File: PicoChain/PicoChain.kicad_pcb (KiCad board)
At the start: 2 copper layers, 14 parts, among them J1 RJ45, J2 RJ45, J3 Conn_01x02_Socket, J4 Conn_01x02_Socket, J5 Conn_01x20_Socket, J6 Conn_01x20_Socket, U1 PCA9615DP, U2 RASPBERRY_PI_PICO

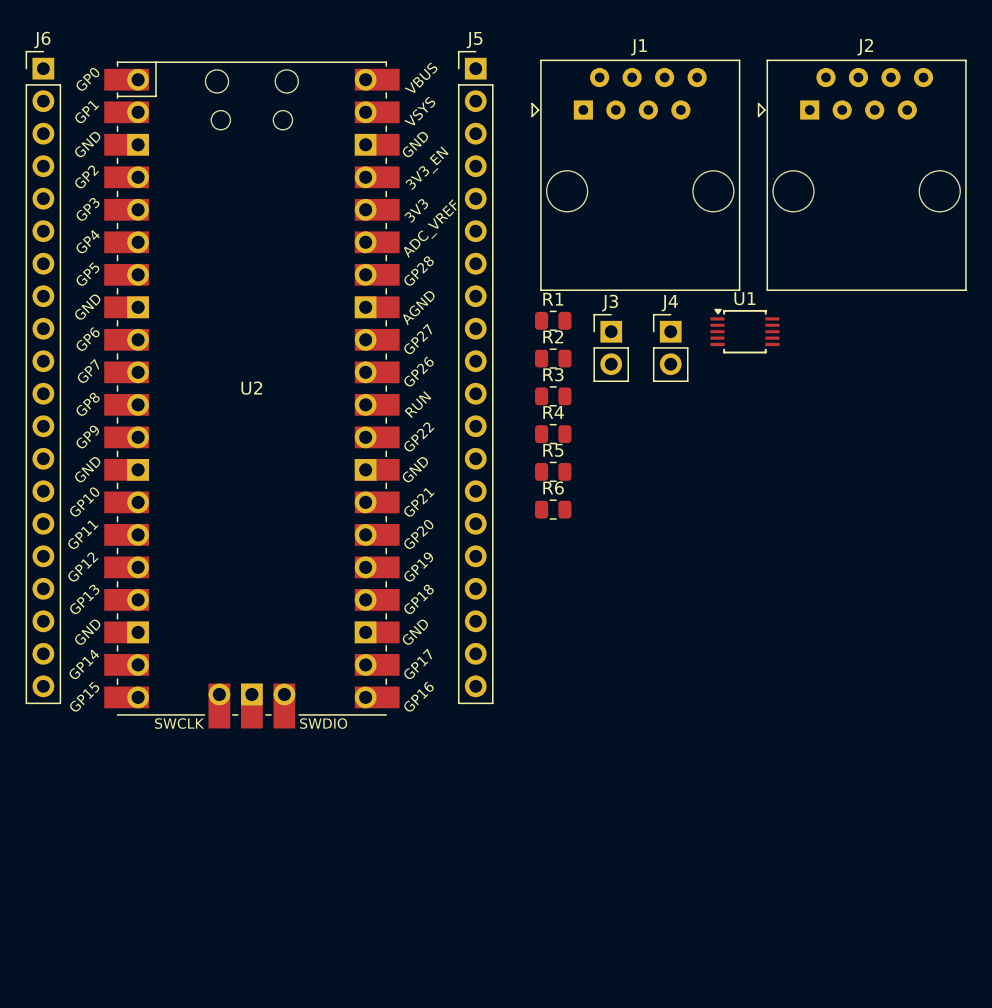
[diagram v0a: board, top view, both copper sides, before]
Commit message: Updated to version 1.1
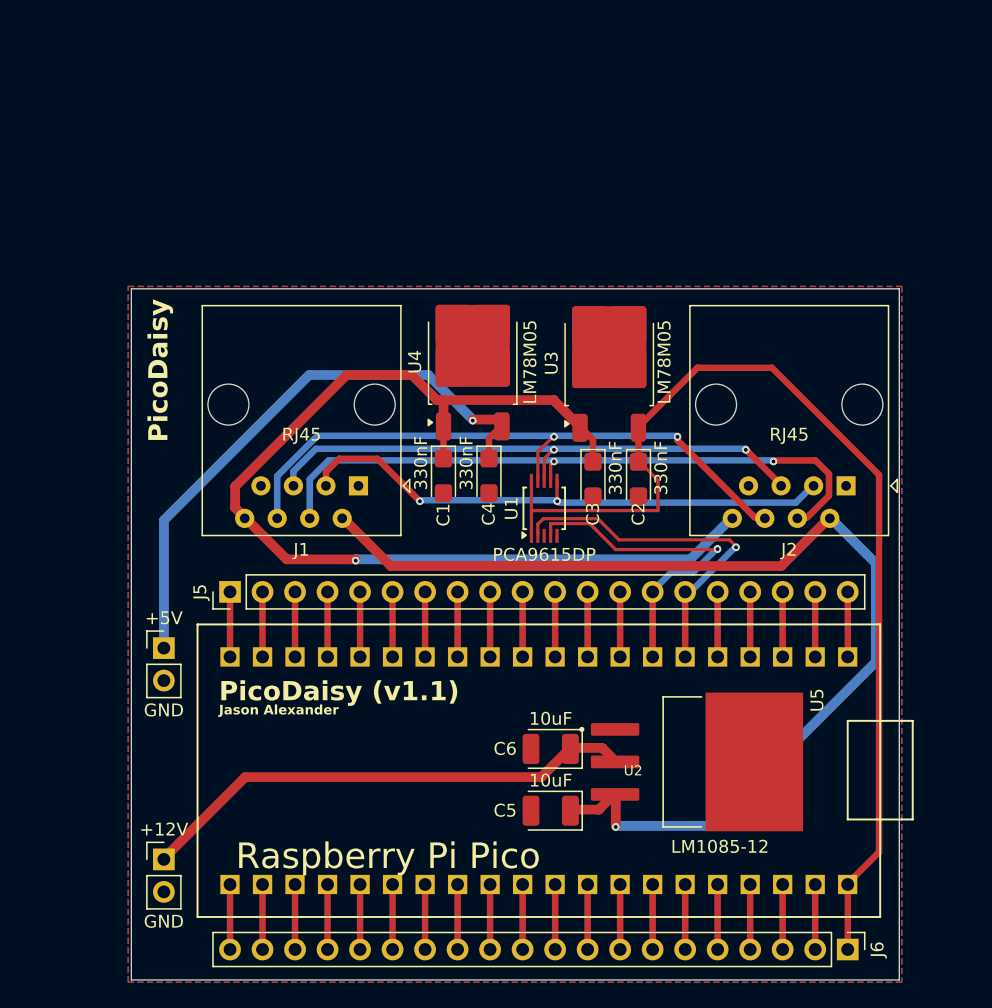
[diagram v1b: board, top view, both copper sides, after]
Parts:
- removed J3, J4: Conn_01x02_Socket, Connector_PinHeader_2.54mm:PinHeader_1x02_P2.54mm_Vertical
- removed R1, R3, R4, R6: 470, Resistor_SMD:R_0805_2012Metric
- removed R2, R5: 140, Resistor_SMD:R_0805_2012Metric
- added +12V: GND, Connector_PinHeader_2.54mm:PinHeader_1x02_P2.54mm_Vertical, F.Cu at (128.5, 112.6)
- added +5V: GND, Connector_PinHeader_2.54mm:PinHeader_1x02_P2.54mm_Vertical, F.Cu at (128.5, 96.1)
- added C1: 330nF, Capacitor_Tantalum_SMD:CP_EIA-3216-18_Kemet-A, F.Cu at (150.4, 82.6)
- added C2: 330nF, Capacitor_Tantalum_SMD:CP_EIA-3216-18_Kemet-A, F.Cu at (165.6, 82.9)
- added C3: 330nF, Capacitor_Tantalum_SMD:CP_EIA-3216-18_Kemet-A, F.Cu at (162.1, 82.9)
- added C4: 330nF, Capacitor_Tantalum_SMD:CP_EIA-3216-18_Kemet-A, F.Cu at (153.9, 82.6)
- added C5: 10uF, Capacitor_Tantalum_SMD:CP_EIA-3528-21_Kemet-B, F.Cu at (158.8, 108.8)
- added C6: 10uF, Capacitor_Tantalum_SMD:CP_EIA-3528-21_Kemet-B, F.Cu at (158.8, 104.0)
- added U3: LM78M05, Package_TO_SOT_SMD:TO-252-2, F.Cu at (163.3, 73.8)
- added U4: LM78M05, Package_TO_SOT_SMD:TO-252-2, F.Cu at (152.7, 73.7)
- added U5: LM1085-12, LM1085IS-12:TO254P1524X483-4N, F.Cu at (170.2, 105.0)
- U2: footprint MCU_RaspberryPi_and_Boards:RPi_Pico_SMD_TH -> RASPBERRY_PI_PICO:RASPBERRY_PI_PICO
- moved J6 93.2 mm to (182.0, 119.6), turned to -90 degrees
- moved J5 45.2 mm to (133.7, 91.7), turned to 90 degrees
- moved U2 38.1 mm to (159.1, 105.7), turned to -90 degrees
- moved J1 34.2 mm to (143.7, 83.4), turned to 180 degrees
- moved J2 29.5 mm to (181.8, 83.4), turned to 180 degrees
- moved U1 20.9 mm to (158.3, 85.2), turned to 90 degrees
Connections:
- J1 pad 1: Net-(U1-DSCLM) -> GND
- J1 pad 2: Net-(U1-DSCLP) -> +24V
- J1 pad 3: +5V -> Net-(U1-DSCLM)
- J1 pad 4: GND -> Net-(U1-DSCLP)
- J1 pad 5: /+5V(M) -> Net-(U1-DSDAP)
- J1 pad 6: +12V -> Net-(U1-DSDAM)
- J1 pad 7: Net-(U1-DSDAM) -> GND
- J1 pad 8: Net-(U1-DSDAP) -> +12V
- J2 pad 1: Net-(U1-DSCLM) -> GND
- J2 pad 2: Net-(U1-DSCLP) -> +24V
- J2 pad 3: +5V -> Net-(U1-DSCLM)
- J2 pad 4: GND -> Net-(U1-DSCLP)
- J2 pad 5: /+5V(M) -> Net-(U1-DSDAP)
- J2 pad 6: +12V -> Net-(U1-DSDAM)
- J2 pad 7: Net-(U1-DSDAM) -> GND
- J2 pad 8: Net-(U1-DSDAP) -> +12V
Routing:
- net +24V: track 0.00 -> 86.2 mm, vias 0 -> 1
- net +5V: track 0.00 -> 84.0 mm
- net +12V: track 0.00 -> 83.4 mm, vias 0 -> 1
- net Net-(U1-DSCLP): track 0.00 -> 50.7 mm, vias 0 -> 2
- net Net-(U1-DSDAM): track 0.00 -> 49.9 mm, vias 0 -> 2
- net /+5V(M): track 0.00 -> 45.6 mm, vias 0 -> 1
- net Net-(U1-DSDAP): track 0.00 -> 43.9 mm, vias 0 -> 2
- net Net-(U1-DSCLM): track 0.00 -> 43.2 mm, vias 0 -> 2
- net /+12V(R): track 0.00 -> 39.3 mm
- net Net-(J5-Pin_15): track 0.00 -> 27.9 mm, vias 0 -> 1
- net Net-(J5-Pin_14): track 0.00 -> 26.3 mm, vias 0 -> 1
- net Net-(J6-Pin_9): track 0.00 -> 5.08 mm
- net Net-(J6-Pin_8): track 0.00 -> 5.08 mm
- net Net-(J6-Pin_7): track 0.00 -> 5.08 mm
- net Net-(J6-Pin_6): track 0.00 -> 5.08 mm
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- added copper zone on B.Cu, net GND
- added copper zone on F.Cu, net GND
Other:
- board outline added: 60 x 54 mm
- board text added: "Jason Alexander"
- board text added: "PicoDaisy"
- board text added: "PicoDaisy (v1.1)"
